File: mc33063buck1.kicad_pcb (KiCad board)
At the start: 2 copper layers, 87.2 x 49 mm, 30 parts, among them J1 Conn_01x01, J2 Conn_01x01, J3 Conn_01x01, J4 USB_A, J5 Jack-DC, Q1 MJE3055T, U1 MC34063

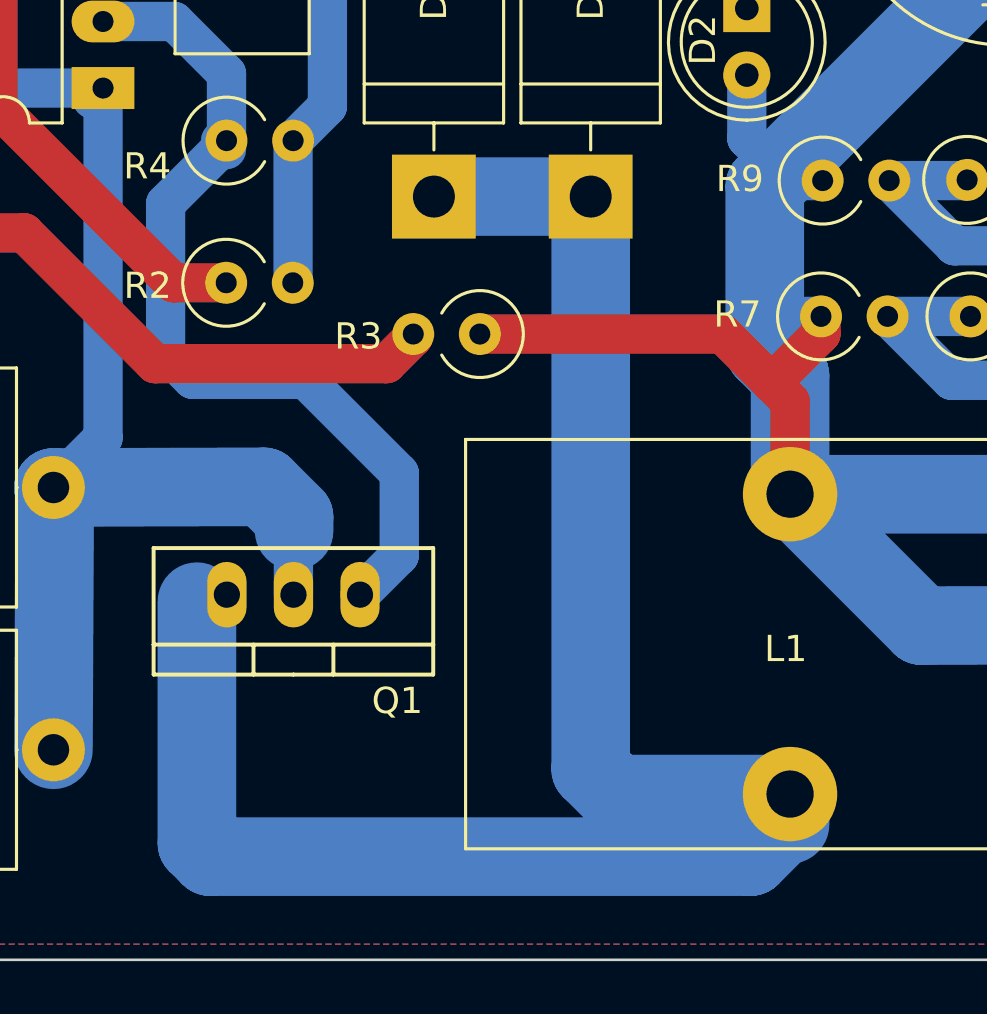
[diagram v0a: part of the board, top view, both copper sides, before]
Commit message: update.
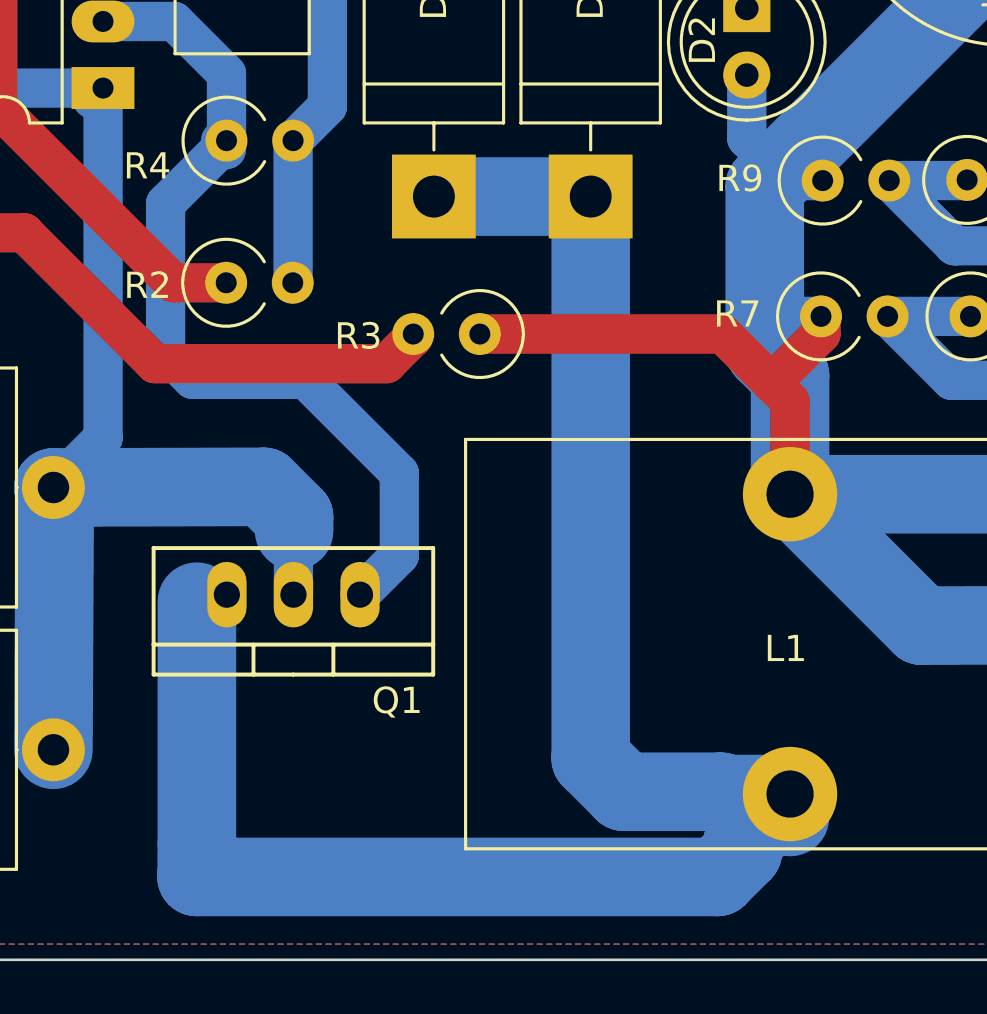
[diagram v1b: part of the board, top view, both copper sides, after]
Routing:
- net Net-(D1-Pad1): track 70.9 -> 71.5 mm
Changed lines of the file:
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@@
-(kicad_pcb (version 4) (host pcbnew 4.0.7)
+(kicad_pcb (version 20171130) (host pcbnew "(5.0.0)")
   (general
-    (links 47)
-    (no_connects 0)
-    (area 1.837157 18.127 114.063043 69.222)
     (thickness 1.6)
     (drawings 4)
-    (tracks 173)
+    (tracks 176)
     (zones 0)
     (modules 30)
@@
   )
   (setup
-    (last_trace_width 1.5)
+    (last_trace_width 0.25)
     (user_trace_width 1.5)
     (user_trace_width 2)
@@
     (visible_elements 7FFFFFFF)
     (pcbplotparams
-      (layerselection 0x010f0_80000001)
+      (layerselection 0x010f0_ffffffff)
       (usegerberextensions false)
       (usegerberattributes true)
+      (usegerberadvancedattributes false)
+      (creategerberjobfile false)
       (excludeedgelayer false)
       (linewidth 0.150000)
@@
       (hpglpennumber 1)
       (hpglpenspeed 20)
-      (hpglpendiameter 15)
-      (hpglpenoverlay 2)
+      (hpglpendiameter 15.000000)
       (psnegative false)
       (psa4output false)
@@
       (net 9 "Net-(J4-Pad5)"))
     (model ${KISYS3DMOD}/Connectors.3dshapes/USB_A.wrl
-      (at (xyz 0.14 0 0))
+      (offset (xyz 3.555999946594238 0 0))
       (scale (xyz 1 1 1))
       (rotate (xyz 0 0 90))
@@
   (segment (start 45.0723 29.5783) (end 36.3855 29.5783) (width 1.5) (layer B.Cu) (net 4))
   (segment (start 36.3855 29.5783) (end 36.0807 29.2735) (width 1.5) (layer B.Cu) (net 4))
-  (segment (start 78.9051 61.595) (end 78.9051 62.4713) (width 3) (layer B.Cu) (net 5))
-  (segment (start 78.9051 62.4713) (end 77.3938 63.9826) (width 3) (layer B.Cu) (net 5))
-  (segment (start 56.2737 63.4746) (end 56.2737 54.2544) (width 3) (layer B.Cu) (net 5))
-  (segment (start 56.7817 63.9826) (end 56.2737 63.4746) (width 3) (layer B.Cu) (net 5))
-  (segment (start 77.3938 63.9826) (end 56.7817 63.9826) (width 3) (layer B.Cu) (net 5))
-  (segment (start 78.9051 61.595) (end 78.9051 62.7507) (width 3) (layer B.Cu) (net 5))
-  (segment (start 71.2978 38.7985) (end 71.2978 60.6425) (width 3) (layer B.Cu) (net 5))
-  (segment (start 72.2503 61.595) (end 78.9051 61.595) (width 3) (layer B.Cu) (net 5))
-  (segment (start 71.2978 60.6425) (end 72.2503 61.595) (width 3) (layer B.Cu) (net 5))
   (segment (start 71.2978 38.7985) (end 71.2978 38.8366) (width 3) (layer B.Cu) (net 5))
   (segment (start 57.4167 53.9877) (end 57.4167 54.3052) (width 1.5) (layer B.Cu) (net 5))
   (segment (start 65.3161 38.7985) (end 71.2978 38.7985) (width 3) (layer B.Cu) (net 5))
+  (segment (start 56.2737 63.4746) (end 56.2737 54.2544) (width 3) (layer B.Cu) (net 5))
+  (segment (start 56.261 64.7573) (end 56.2737 63.4746) (width 3) (layer B.Cu) (net 5))
+  (segment (start 78.9051 61.595) (end 78.9051 62.4713) (width 3) (layer B.Cu) (net 5))
+  (segment (start 77.105101 63.394999) (end 77.105101 63.788699) (width 3) (layer B.Cu) (net 5))
+  (segment (start 78.9051 61.595) (end 77.105101 63.394999) (width 3) (layer B.Cu) (net 5))
+  (segment (start 76.1365 64.7573) (end 56.261 64.7573) (width 3) (layer B.Cu) (net 5))
+  (segment (start 77.105101 63.788699) (end 76.1365 64.7573) (width 3) (layer B.Cu) (net 5))
+  (segment (start 76.359516 61.595) (end 76.270616 61.5061) (width 3) (layer B.Cu) (net 5))
+  (segment (start 78.9051 61.595) (end 76.359516 61.595) (width 3) (layer B.Cu) (net 5))
+  (segment (start 76.270616 61.5061) (end 72.5678 61.5061) (width 3) (layer B.Cu) (net 5))
+  (segment (start 71.2978 60.2361) (end 71.2978 38.7985) (width 3) (layer B.Cu) (net 5))
+  (segment (start 72.5678 61.5061) (end 71.2978 60.2361) (width 3) (layer B.Cu) (net 5))
   (segment (start 77.2541 31.623) (end 77.2541 27.2034) (width 1.5) (layer B.Cu) (net 6))
   (segment (start 77.2541 27.2034) (end 77.3303 27.1272) (width 1.5) (layer B.Cu) (net 6))
